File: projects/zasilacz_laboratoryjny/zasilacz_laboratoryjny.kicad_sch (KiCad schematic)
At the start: 33 parts, among them J1 Conn_Point, J2 Conn_Point, J3 Conn_Point, J4 Conn_Point, P1 10kΩ, T1 BC557, T2 BC557, T3 BC547, T4 BC547, T5 BC557, U1 DB207, U2 LM317, U3 Voltmeter_digital, Y1 Buzzer_Piezo_Active

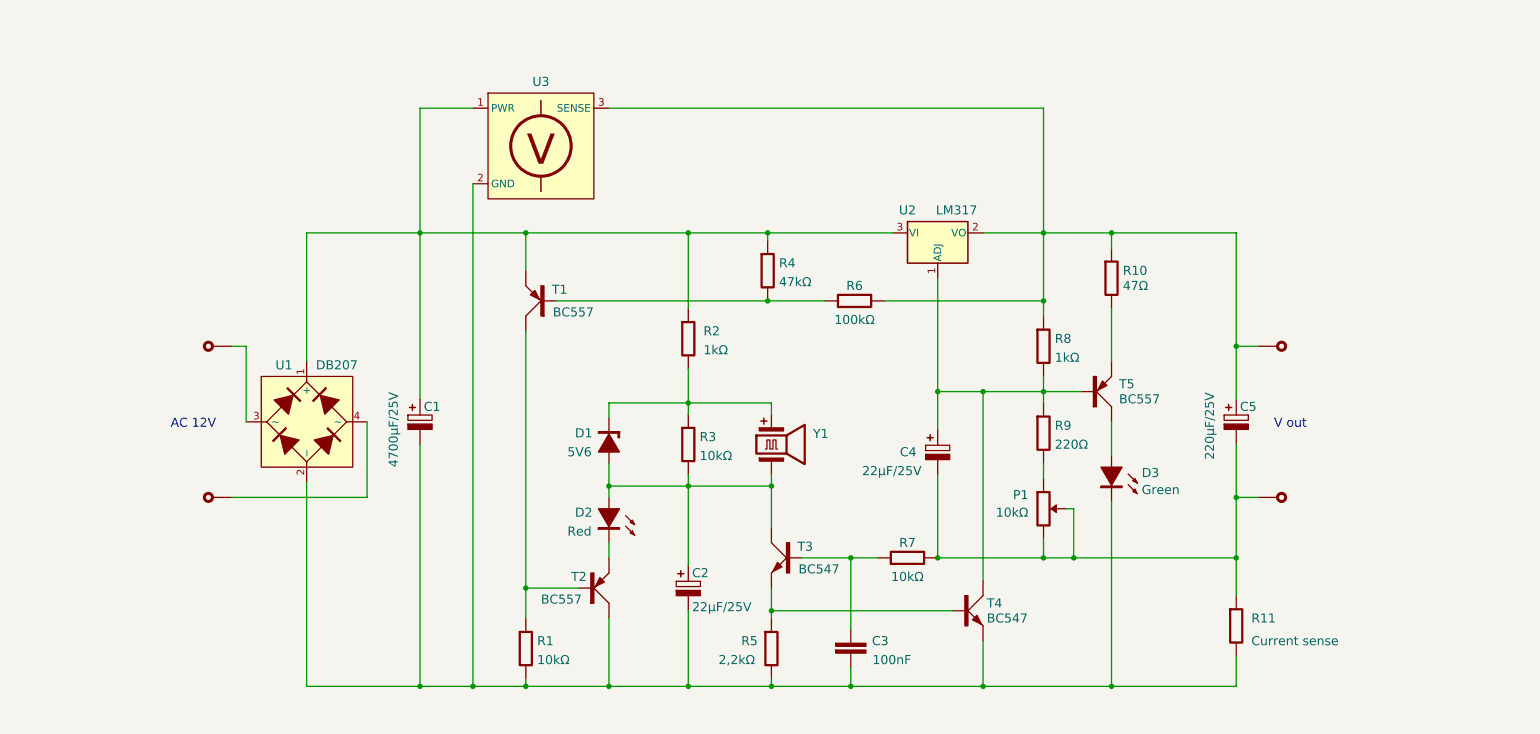
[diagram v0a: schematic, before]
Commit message: zasilacz laboratoryjny v2.0
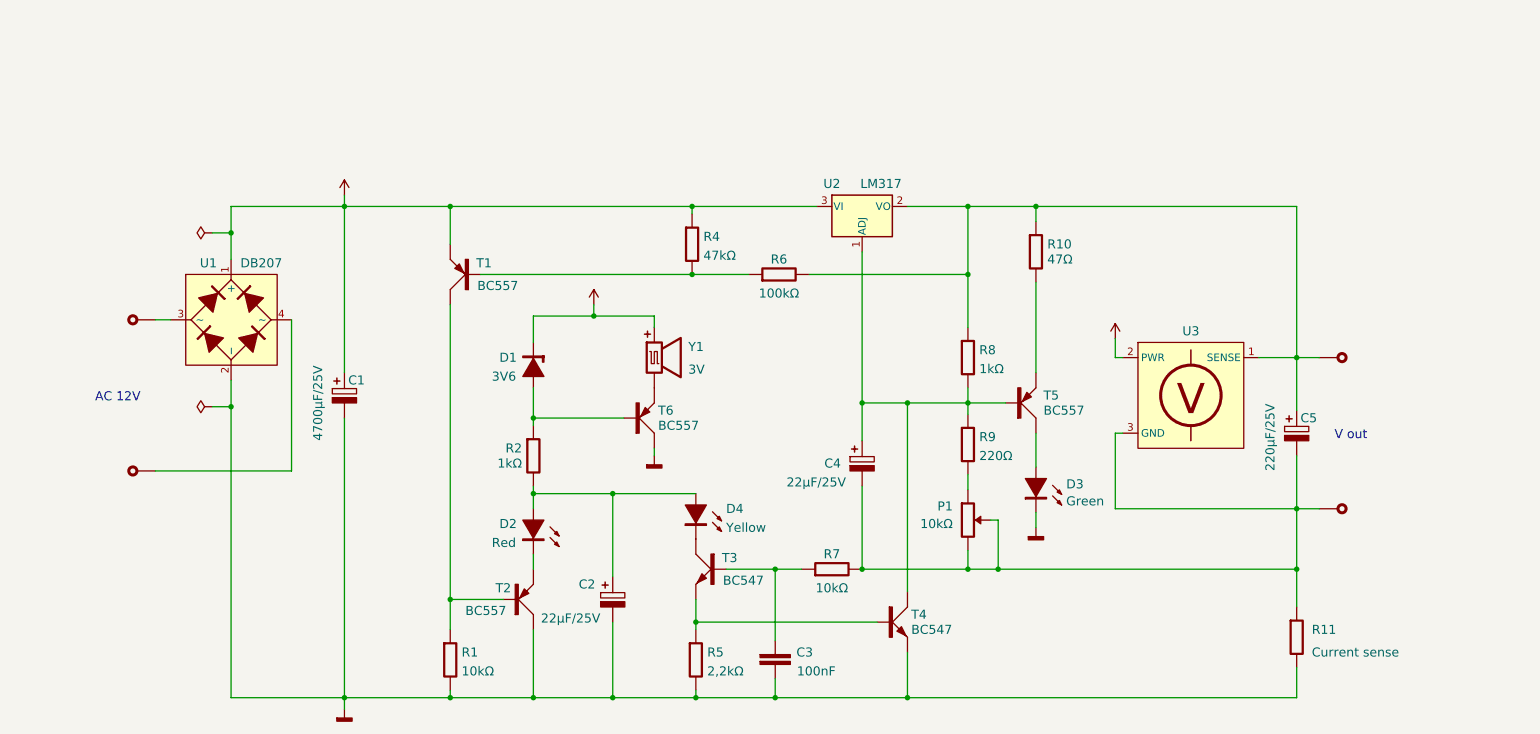
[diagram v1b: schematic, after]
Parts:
- removed R3: 10kΩ, symbol *Custom_Generic:R
- removed Y1: Buzzer_Piezo_Active, symbol *Custom_Generic:Buzzer_Piezo_Active
- added D4: Yellow, symbol *Custom_Generic:LED
- added T6: BC557, symbol *Custom_Generic:PNP_BJT_BCE
- added Y1: 3V, symbol *Custom_Generic:Buzzer_Magnetic_Active
- D1: value 5V6 -> 3V6
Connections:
- net GNDD: now reaches C1.1 (-), C2.1 (-), C3.2, D3.1 (K), R1.2, R11.2, R5.2, T2.2 (C), T4.3 (E), U1.2 (−)
- net GNDD: now also T6.2 (C); no longer U3.2 (GND)
- net VDC: now reaches C1.2 (+), R4.1, T1.3 (E), U1.1 (+), U2.3 (VI)
- net VDC: now also D1.1 (K), U3.2 (PWR), Y1.1; no longer R2.1, U3.1 (PWR)
- net at C2.2 (+), D2.2 (A): now also R2.2, D4.2 (A); no longer D1.2 (A), T3.1 (C)
- net at C5.2 (+), J3.1 (Pin_1), R10.1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: now also U3.1 (SENSE); no longer U3.3 (SENSE)
- net at C4.1 (-), C5.1 (-), J4.1 (Pin_1)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: now also U3.3 (GND)
- new net: T6.3 (E), Y1.2
- new net: D1.2 (A), R2.1, T6.1 (B)
- new net: D4.1 (K), T3.1 (C)
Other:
- moved on the sheet: C1, C2, C3, C4, C5, D1, D2, D3, P1, R1, R10, R11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

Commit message: Wersja 2.0 po modyfikacjach wynikłych z testowania
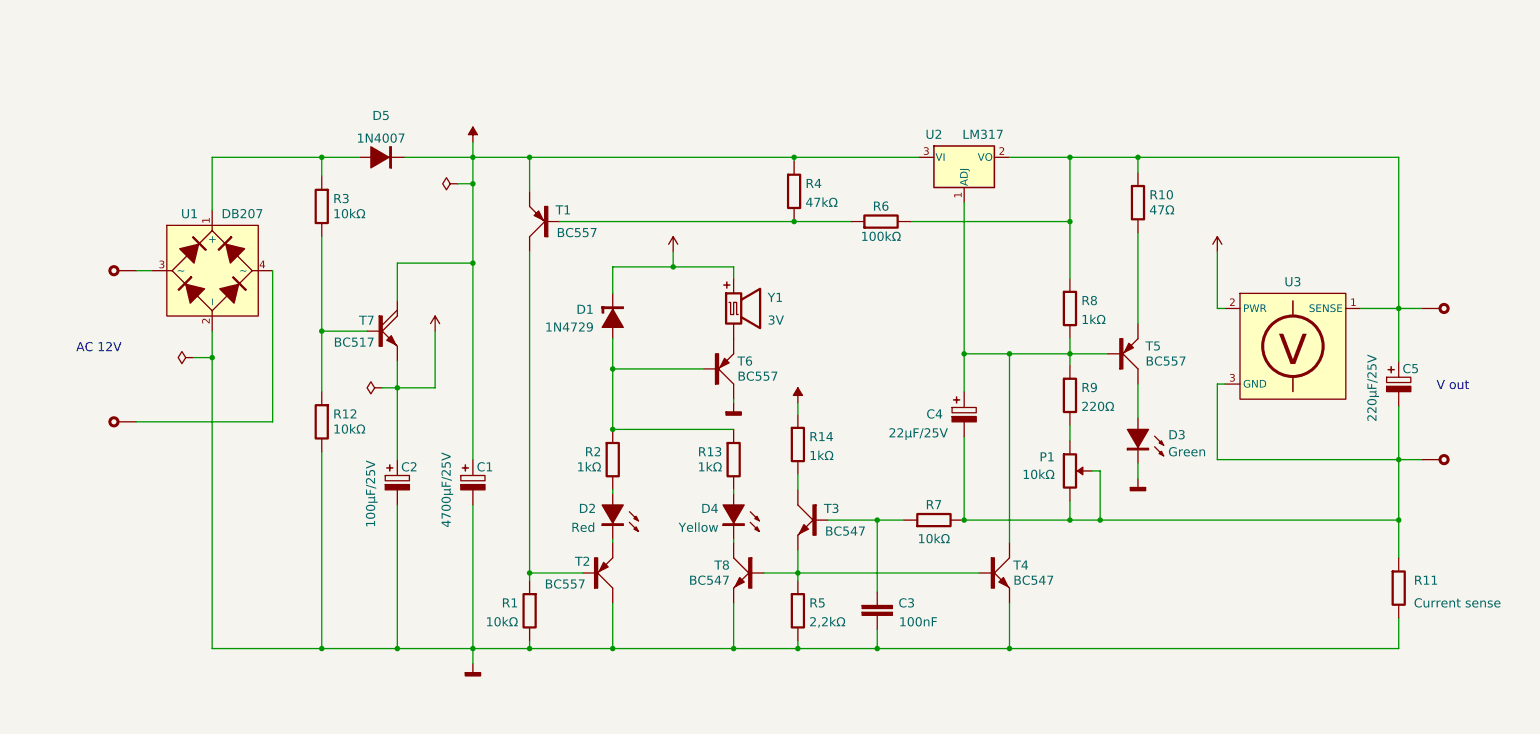
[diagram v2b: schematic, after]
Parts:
- added D5: 1N4007, symbol *Custom_Generic:D
- added R12, R3: 10kΩ, symbol *Custom_Generic:R
- added R13, R14: 1kΩ, symbol *Custom_Generic:R
- added T7: BC517, symbol *Custom_Generic:NPN_Darlington_CBE
- added T8: BC547, symbol *Custom_Generic:NPN_BJT_CBE
- C2: value 22μF/25V -> 100μF/25V
- D1: value 3V6 -> 1N4729
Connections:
- net at D2.2 (A), R2.2: no longer C2.2 (+), D4.2 (A)
- net at D1.2 (A), R2.1, T6.1 (B): now also R13.1
- net at R5.1, T3.3 (E), T4.2 (B): now also T8.2 (B)
- net at D4.1 (K): now also T8.1 (C); no longer T3.1 (C)
- net GNDD renamed GND
- net GND: now also R12.2, T8.3 (E)
- net VDC renamed V1
- net V1: now also D5.1 (K), R14.1, T7.1 (C); no longer D1.1 (K), U1.1 (+), U3.2 (PWR), Y1.1
- new net: D4.2 (A), R13.2
- new net: D5.2 (A), R3.1, U1.1 (+)
- new net: R12.1, R3.2, T7.2 (B)
- new net: R14.2, T3.1 (C)
- new net V3: C2.2 (+), D1.1 (K), T7.3 (E), U3.2 (PWR), Y1.1
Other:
- moved on the sheet: C1, C3, C4, C5, D1, D2, D3, D4, P1, R1, R10, R11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

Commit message: preparations for board design in VeeCAD
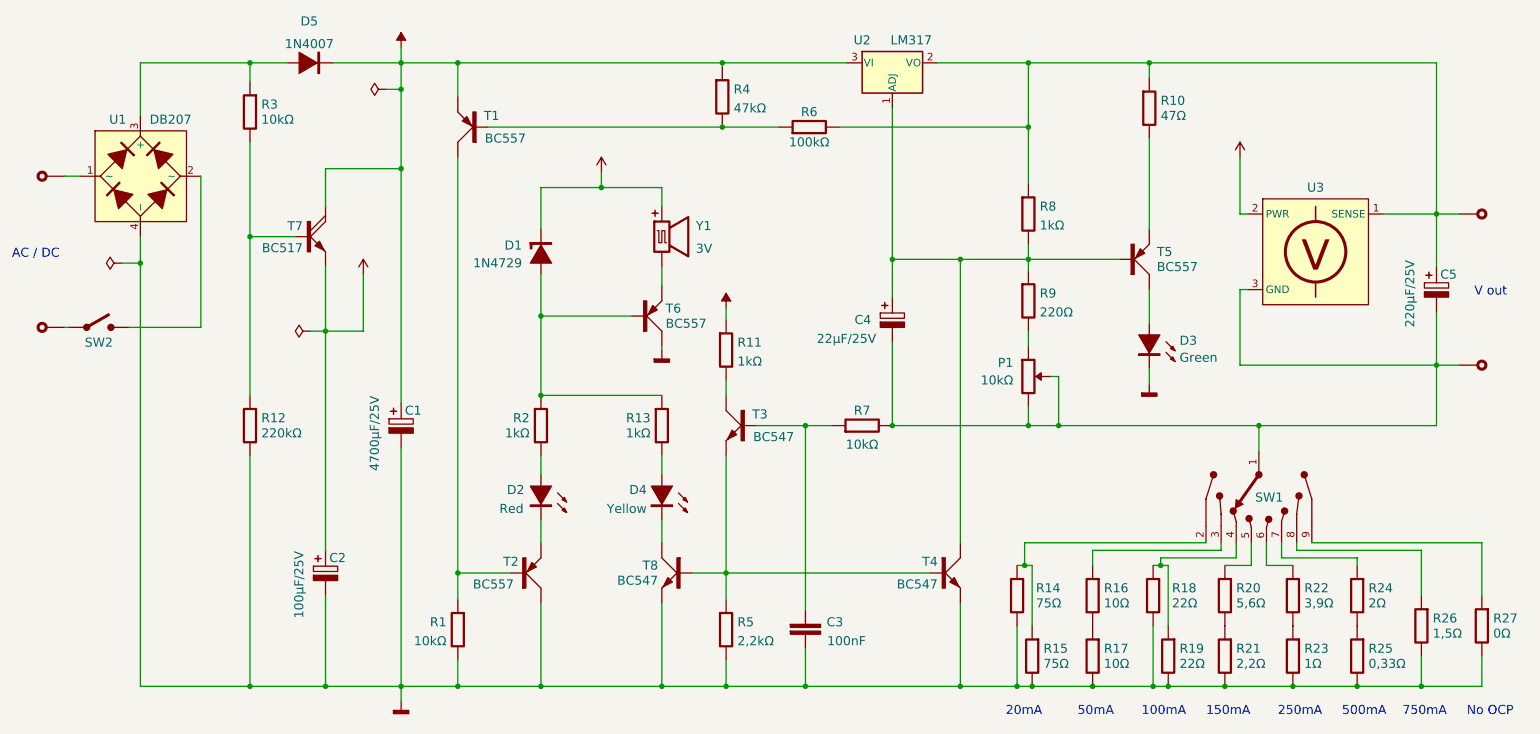
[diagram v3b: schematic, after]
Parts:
- removed R11: Current sense, symbol *Custom_Generic:R
- added R14, R15: 75Ω, VeeCad:AX3_1N, symbol *Custom_Generic:R
- added R16, R17: 10Ω, VeeCad:AX3_1N, symbol *Custom_Generic:R
- added R18, R19: 22Ω, VeeCad:AX3_1N, symbol *Custom_Generic:R
- added R20: 5,6Ω, VeeCad:AX3_1N, symbol *Custom_Generic:R
- added R21: 2,2Ω, VeeCad:AX3_1N, symbol *Custom_Generic:R
- added R22: 3,9Ω, VeeCad:AX6_2N, symbol *Custom_Generic:R
- added R23: 1Ω, VeeCad:AX6_2N, symbol *Custom_Generic:R
- added R24: 2Ω, VeeCad:AX6_2N, symbol *Custom_Generic:R
- added R25: 0,33Ω, VeeCad:AX6_2N, symbol *Custom_Generic:R
- added R26: 1,5Ω, VeeCad:AX6_2N, symbol *Custom_Generic:R
- added R27: 0Ω, VeeCad:AX1_1N, symbol *Custom_Generic:R
- added SW1: SW_SP8T, VeeCad:SIP9, symbol *Custom_Generic:SW_SP8T
- added SW2: SW_SPST, VeeCad:SIP2, symbol *Custom_Generic:SW_SPST
- C1: footprint (none) -> VeeCad:RA3_6
- C2, C4: footprint (none) -> VeeCad:RA1_2
- C3: footprint (none) -> VeeCad:AX2_1N
- C5: footprint (none) -> VeeCad:RA1_3
- D1, D5: footprint (none) -> VeeCad:AX2_1
- D2, D3, D4: footprint (none) -> VeeCad:SIP2
- J1, J2, J3, J4: footprint (none) -> VeeCad:SIP1
- P1, U3: footprint (none) -> VeeCad:SIP3
- R1, R10, R13, R2, R3, R4, R5, R6, R7, R8, R9: footprint (none) -> VeeCad:AX3_1N
- R11: renamed from R14; footprint (none) -> VeeCad:AX3_1N
- R12: value 10kΩ -> 220kΩ; footprint (none) -> VeeCad:AX3_1N
- T1, T2, T3, T4, T5, T6, T7, T8: footprint (none) -> VeeCad:TO92
- U1: footprint (none) -> VeeCad:DIP4_6
- U2: footprint Package_TO_SOT_THT:TO-220-3_Vertical -> VeeCad:TO220
- Y1: footprint (none) -> VeeCad:BUZR_12
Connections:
- net GND: now also U1.4 (−), R14.2, R15.2, R17.2, R18.2, R19.2, R21.2, R23.2, R25.2, R26.2, R27.2; no longer U1.2 (−)
- net at C4.1 (-), C5.1 (-), J4.1 (Pin_1)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: now also SW1.1
- net at D5.2 (A), R3.1: now also U1.3 (+); no longer U1.1 (+)
- net at J2.1 (Pin_1): now also SW2.2 (B1); no longer U1.4 (∼)
- net at J1.1 (Pin_1): now also U1.1 (∼); no longer U1.3 (∼)
- new net: R20.1, SW1.5
- new net: R20.2, R21.1
- new net: R27.1, SW1.9
- new net: R18.1, R19.1, SW1.4
- new net: R14.1, R15.1, SW1.2
- new net: SW2.1 (A1), U1.2 (∼)
- new net: R24.1, SW1.7
- new net: R24.2, R25.1
- new net: R22.1, SW1.6
- new net: R22.2, R23.1
- new net: R26.1, SW1.8
- new net: R16.2, R17.1
- new net: R16.1, SW1.3
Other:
- note added: "100mA"
- note added: "150mA"
- note added: "20mA"
- note added: "250mA"
- note added: "500mA"
- note added: "50mA"
- note added: "750mA"
- note added: "AC / DC"
- note added: "No OCP"
- note removed: "AC 12V"
- moved on the sheet: C1, C2, C3, C4, C5, D1, D2, D3, D4, D5, P1, R1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
